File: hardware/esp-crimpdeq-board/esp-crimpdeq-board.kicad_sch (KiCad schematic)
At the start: 72 parts, among them J1 USB4105-GF-A, J2 Conn_01x02_Pin, Q1 DMG3415U, SW1 SW_Push, SW2 SW_Push, U1 SHTC3, U2 ICM-42670-P, U3 REF35330QDBVR, U4 SY8088, U5 NAU7802SGI, U6 MCP73831T-2ACI/OT, U7 MAX17262, U8 ESP32-C6-MINI-1/U, Y1 32.768Hz

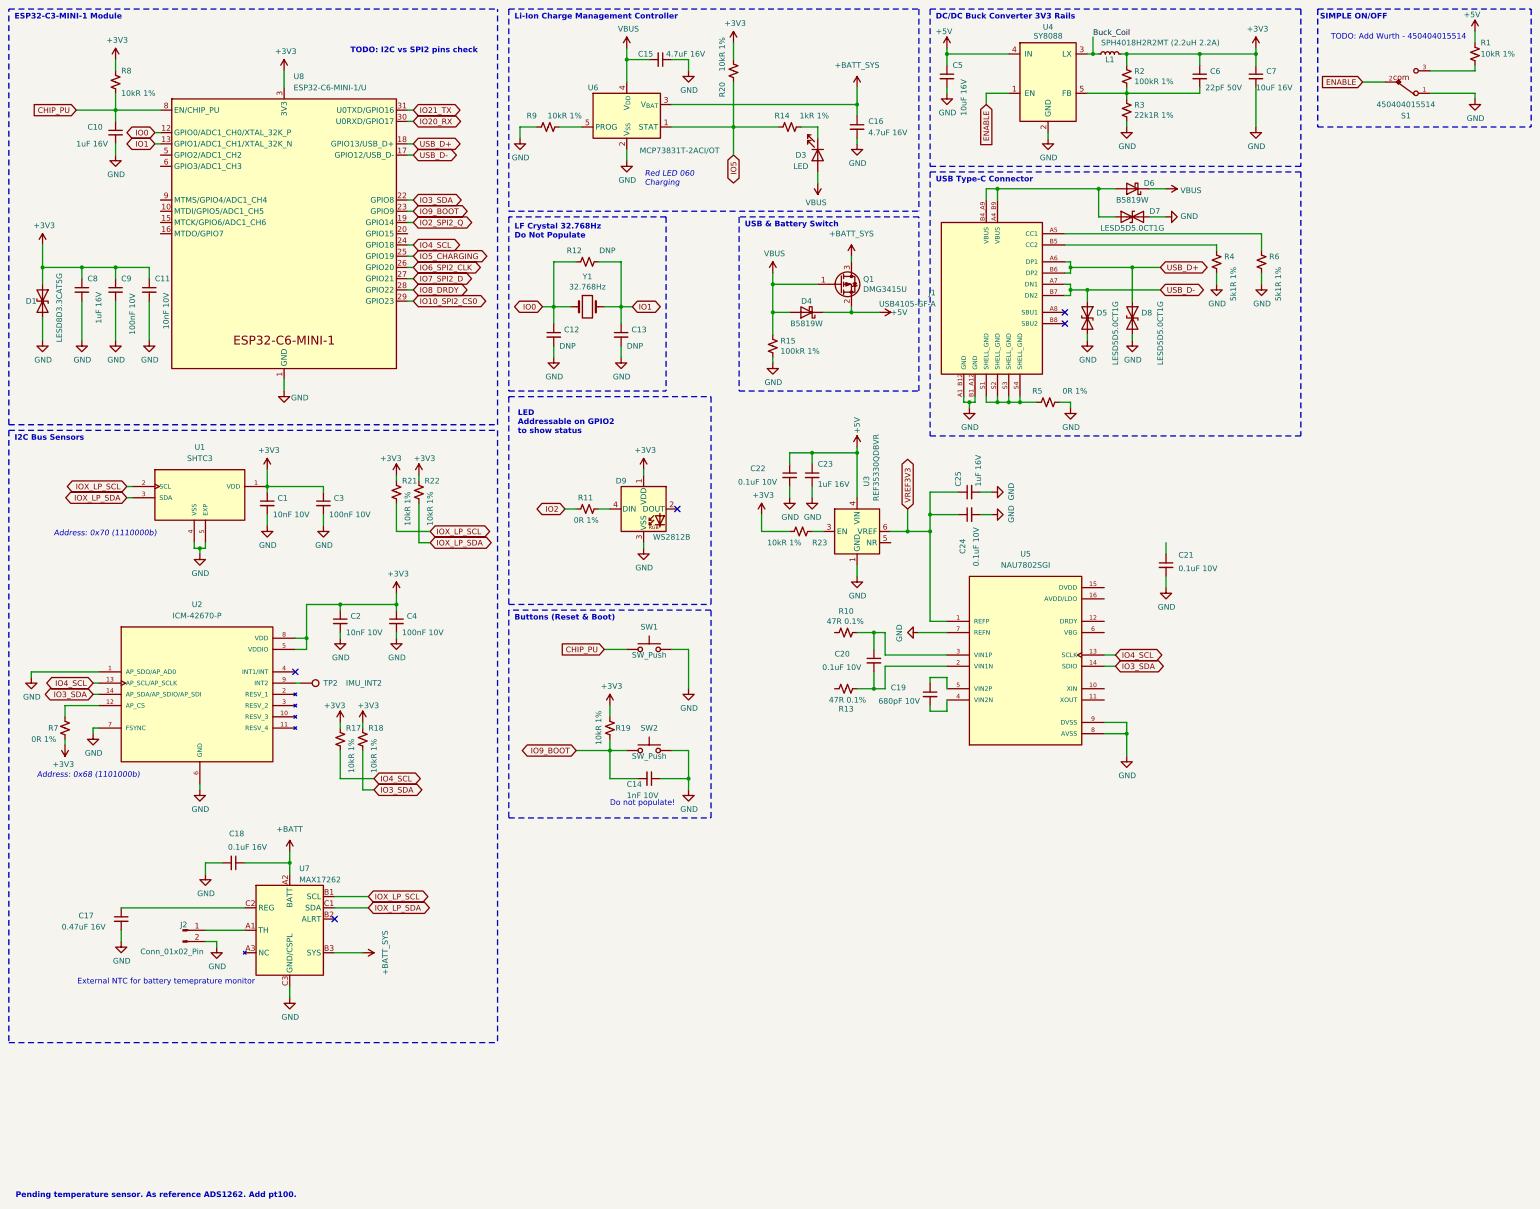
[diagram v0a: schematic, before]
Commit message: Update esp-crimpdeq-board.kicad_sch
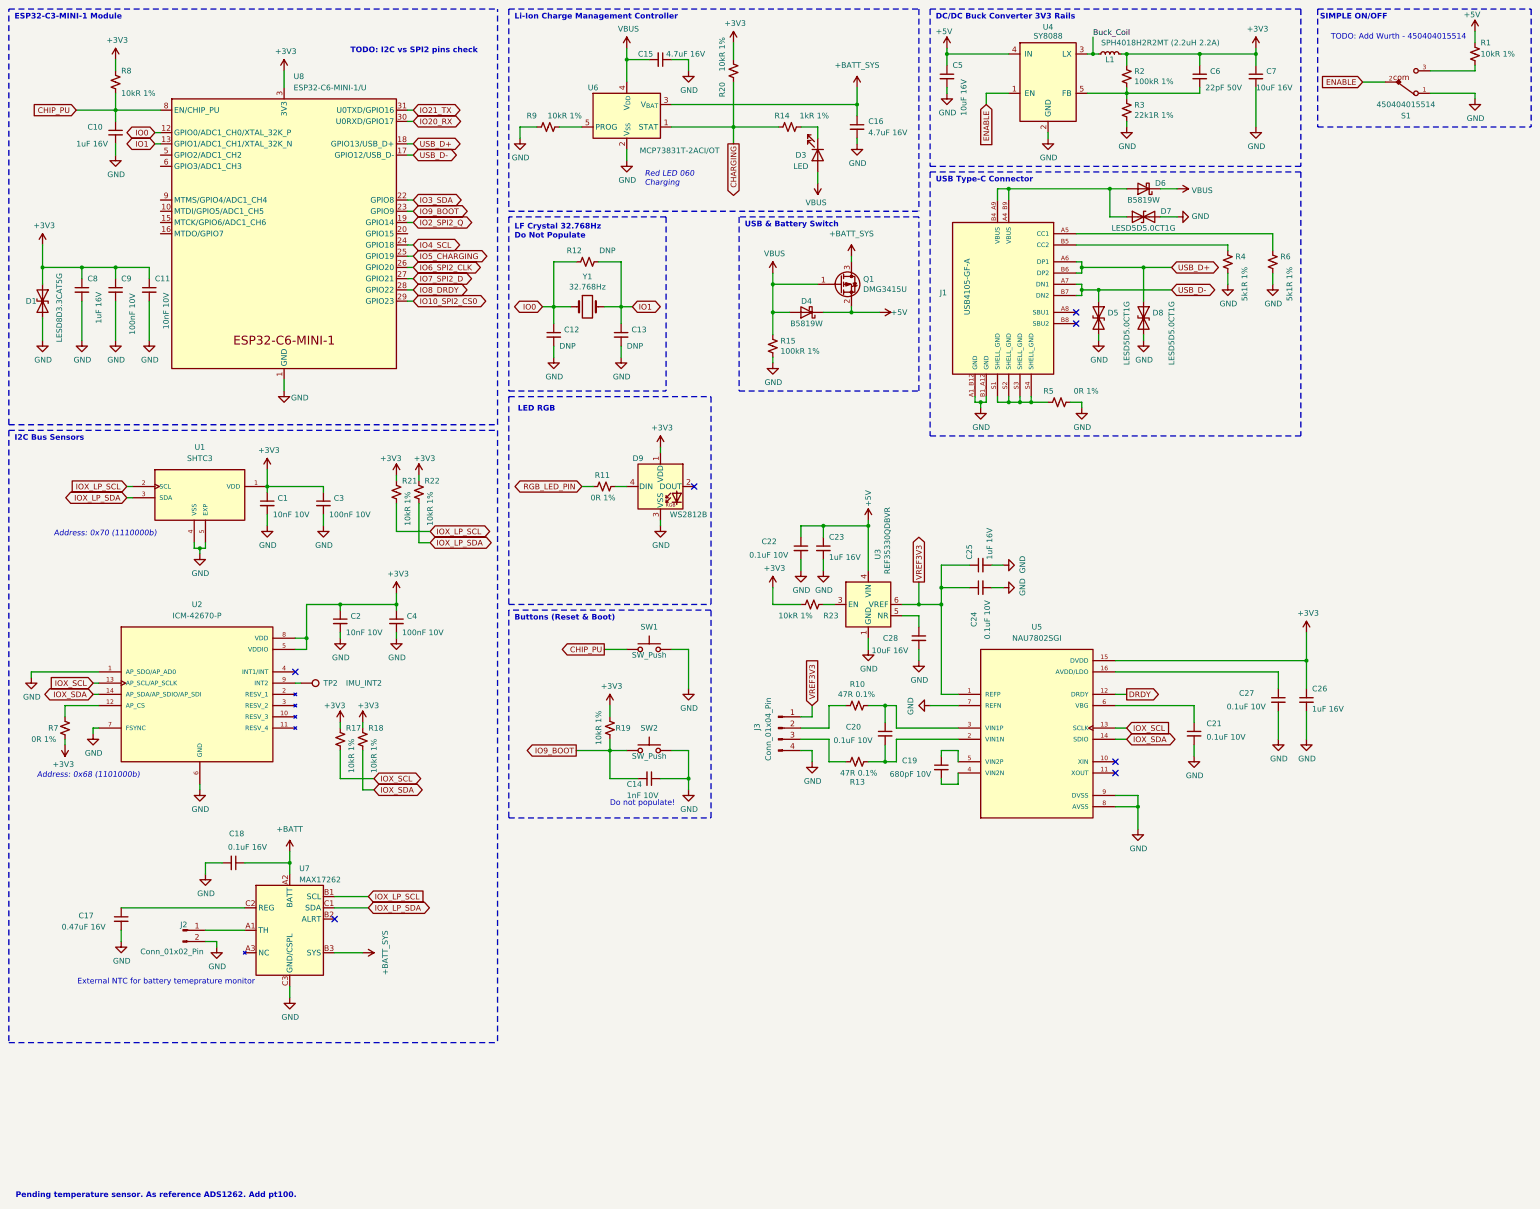
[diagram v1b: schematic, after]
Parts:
- removed U5: NAU7802SGI, Package_SO:SOP-16_3.9x9.9mm_P1.27mm, symbol Nuvoton:NAU7802SGI
- added C26: 1uF 16V, Capacitor_SMD:C_0402_1005Metric, symbol Device:C_Small
- added C27: 0.1uF 10V, Capacitor_SMD:C_0402_1005Metric, symbol Device:C_Small
- added C28: 10uF 16V, Capacitor_SMD:C_0805_2012Metric, symbol Device:C_Small
- added J3: Conn_01x04_Pin, Connector_PinHeader_1.27mm:PinHeader_1x04_P1.27mm_Vertical, symbol Connector:Conn_01x04_Pin
- added U5: NAU7802SGI, Package_SO:SOP-16_3.9x9.9mm_P1.27mm, symbol PCM_Nuvoton:NAU7802SGI
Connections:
- net +3V3: now also C26.1, U5.15 (DVDD)
- net GND: now also C26.2, C27.2, C28.2, J3.4 (Pin_4), U5.7 (REFN), U5.8 (AVSS), U5.9 (DVSS)
- net IO3_SDA: no longer R18.2, U2.14 (AP_SDA/AP_SDIO/AP_SDI)
- net IO4_SCL: no longer R17.2, U2.13 (AP_SCL/AP_SCLK)
- net VREF3V3: now also J3.1 (Pin_1), U5.1 (REFP)
- net at C21.1: now also U5.6 (VBG)
- net at C19.1: now also U5.5 (VIN2P)
- net at C19.2: now also U5.4 (VIN2N)
- net at R13.1: now also J3.3 (Pin_3)
- net at C20.2, R13.2: now also U5.2 (VIN1N)
- net at U3.5 (NR): now also C28.1
- net at C20.1, R10.2: now also U5.3 (VIN1P)
- net at R10.1: now also J3.2 (Pin_2)
- net IO2 renamed RGB_LED_PIN
- net IO5 renamed CHARGING
- new net: C27.1, U5.16 (AVDD/LDO)
- new net DRDY: U5.12 (DRDY)
- new net IOX_SCL: R17.2, U2.13 (AP_SCL/AP_SCLK), U5.13 (SCLK)
- new net IOX_SDA: R18.2, U2.14 (AP_SDA/AP_SDIO/AP_SDI), U5.14 (SDIO)
- no-connect marks 5 -> 7
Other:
- note added: "LED RGB"
- note removed: "LED Addressable on GPIO2 to show status"
- moved on the sheet: C19, C20, C21, C22, C23, C24, C25, D5, D6, D7, D8, D9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
